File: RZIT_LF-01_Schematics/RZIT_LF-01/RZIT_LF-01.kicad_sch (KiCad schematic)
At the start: 0 parts

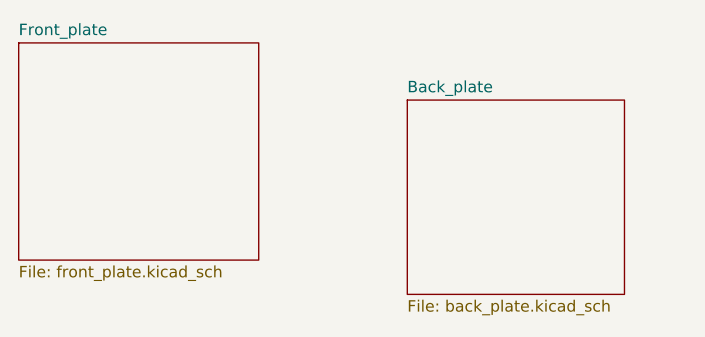
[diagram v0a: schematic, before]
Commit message: Changes
addetd
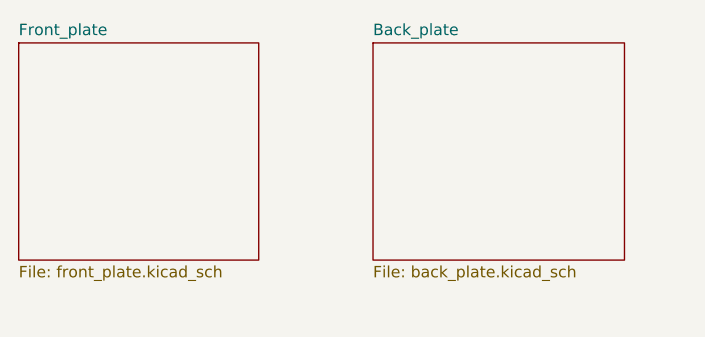
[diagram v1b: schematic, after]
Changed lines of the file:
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@@
 (kicad_sch (version 20211123) (generator eeschema)
   (paper "A4")
-  (sheet (at 118.11 54.61) (size 24.13 21.59) (fields_autoplaced)
+  (sheet (at 114.3 48.26) (size 27.94 24.13) (fields_autoplaced)
     (stroke (width 0.1524) (type solid) (color 0 0 0 0))
     (fill (color 0 0 0 0.0000))
-    (property "Sheet name" "Back_plate" (id 0) (at 118.11 53.8984 0)
+    (property "Sheet name" "Back_plate" (id 0) (at 114.3 47.5484 0)
       (effects (font (size 1.27 1.27)) (justify left bottom))
     )
-    (property "Sheet file" "back_plate.kicad_sch" (id 1) (at 118.11 76.7846 0)
+    (property "Sheet file" "back_plate.kicad_sch" (id 1) (at 114.3 72.9746 0)
       (effects (font (size 1.27 1.27)) (justify left top))
     )
@@
       (reference "#PWR?") (unit 1) (value "GND") (footprint "")
     )
+    (path "/2e1b8e48-0b26-4cf5-b4e7-1ce16b5ce0be/08574ea4-3686-4249-a3df-6a8f55c428f0"
+      (reference "#PWR?") (unit 1) (value "+3.3V") (footprint "")
+    )
     (path "/2e1b8e48-0b26-4cf5-b4e7-1ce16b5ce0be/08fac2eb-8669-4a36-b11c-7892fe3d12e2"
       (reference "#PWR?") (unit 1) (value "GND") (footprint "")
@@
       (reference "#PWR?") (unit 1) (value "+3.3V") (footprint "")
     )
+    (path "/2e1b8e48-0b26-4cf5-b4e7-1ce16b5ce0be/24ba3905-43ac-4e40-82e7-128d44942746"
+      (reference "#PWR?") (unit 1) (value "GND") (footprint "")
+    )
     (path "/2e1b8e48-0b26-4cf5-b4e7-1ce16b5ce0be/25eb344f-2e26-4af0-b9d7-c2dc91bae6a6"
       (reference "#PWR?") (unit 1) (value "GND") (footprint "")
@@
       (reference "#PWR?") (unit 1) (value "+3.3V") (footprint "")
     )
+    (path "/2e1b8e48-0b26-4cf5-b4e7-1ce16b5ce0be/30170b01-1124-4e99-90be-46e160dec4f3"
+      (reference "#PWR?") (unit 1) (value "GND") (footprint "")
+    )
     (path "/2e1b8e48-0b26-4cf5-b4e7-1ce16b5ce0be/31a9cdd2-5288-4d9b-bf4b-95e2dd897f61"
       (reference "#PWR?") (unit 1) (value "+3.3V") (footprint "")
@@
       (reference "#PWR?") (unit 1) (value "+3.3V") (footprint "")
     )
-    (path "/2e1b8e48-0b26-4cf5-b4e7-1ce16b5ce0be/a720cf76-448f-4fa9-b241-862453258760"
-      (reference "#PWR?") (unit 1) (value "GND") (footprint "")
-    )
     (path "/2e1b8e48-0b26-4cf5-b4e7-1ce16b5ce0be/a79bf299-ed19-4f53-9d17-c9f2e158af71"
       (reference "#PWR?") (unit 1) (value "GND") (footprint "")
@@
       (reference "#PWR?") (unit 1) (value "+3.3V") (footprint "")
     )
+    (path "/2e1b8e48-0b26-4cf5-b4e7-1ce16b5ce0be/d7035a7a-77eb-4ac5-a4a7-60dbe8fb1ef1"
+      (reference "C?") (unit 1) (value "100nF") (footprint "")
+    )
+    (path "/2e1b8e48-0b26-4cf5-b4e7-1ce16b5ce0be/f7f08f22-7201-41d0-b3e9-3d6d3862c50b"
+      (reference "C?") (unit 1) (value "4.7uF") (footprint "")
+    )
     (path "/2e1b8e48-0b26-4cf5-b4e7-1ce16b5ce0be/1c2dab5a-9a43-4cc0-b7fa-78917f8390f0"
       (reference "R?") (unit 1) (value "200") (footprint "")
@@
       (reference "R?") (unit 1) (value "20k") (footprint "")
     )
+    (path "/2e1b8e48-0b26-4cf5-b4e7-1ce16b5ce0be/3eee4add-1700-4e59-b90c-0c7ae537c501"
+      (reference "R?") (unit 1) (value "10k") (footprint "")
+    )
     (path "/2e1b8e48-0b26-4cf5-b4e7-1ce16b5ce0be/48d87eda-b5a7-4dd7-8482-e51be96f6a18"
       (reference "R?") (unit 1) (value "20k") (footprint "")
@@
       (reference "R?") (unit 1) (value "20k") (footprint "")
     )
+    (path "/2e1b8e48-0b26-4cf5-b4e7-1ce16b5ce0be/6031abde-b833-4f66-a1d6-40421ab3a37f"
+      (reference "R?") (unit 1) (value "10k") (footprint "")
+    )
     (path "/2e1b8e48-0b26-4cf5-b4e7-1ce16b5ce0be/72bb3040-bd09-4e3a-95bc-d3043bc9b4b7"
       (reference "R?") (unit 1) (value "200") (footprint "")
     )
+    (path "/2e1b8e48-0b26-4cf5-b4e7-1ce16b5ce0be/7ce0890a-dc24-451f-8dc3-ef0f4639c18f"
+      (reference "R?") (unit 1) (value "10k") (footprint "")
+    )
     (path "/2e1b8e48-0b26-4cf5-b4e7-1ce16b5ce0be/80299693-a029-4038-b7d8-5c94f629dc1d"
       (reference "R?") (unit 1) (value "20k") (footprint "")
@@
       (reference "R?") (unit 1) (value "200") (footprint "")
     )
+    (path "/2e1b8e48-0b26-4cf5-b4e7-1ce16b5ce0be/c12a6f96-6f0b-46b9-aaed-d5e718e4d3d6"
+      (reference "R?") (unit 1) (value "10k") (footprint "")
+    )
     (path "/2e1b8e48-0b26-4cf5-b4e7-1ce16b5ce0be/d2a58691-1ce2-4a44-b02d-e07298cb17d6"
       (reference "R?") (unit 1) (value "200") (footprint "")
@@
       (reference "U?") (unit 1) (value "QRE1113") (footprint "OptoDevice:OnSemi_CASE100AQ")
     )
-    (path "/2e1b8e48-0b26-4cf5-b4e7-1ce16b5ce0be/86eab7b8-2ba1-468f-aff8-8d00b048fda5"
+    (path "/2e1b8e48-0b26-4cf5-b4e7-1ce16b5ce0be/94c9a039-9b74-442a-be87-64ea896cb680"
+      (reference "U?") (unit 1) (value "QRE1113") (footprint "OptoDevice:OnSemi_CASE100AQ")
+    )
+    (path "/2e1b8e48-0b26-4cf5-b4e7-1ce16b5ce0be/9fa2dc80-2843-4c91-ad55-e90083707e05"
+      (reference "U?") (unit 1) (value "QRE1113") (footprint "OptoDevice:OnSemi_CASE100AQ")
+    )
+    (path "/2e1b8e48-0b26-4cf5-b4e7-1ce16b5ce0be/aac6220a-eaf7-46a5-9ea8-0cbd9e35573d"
+      (reference "U?") (unit 1) (value "QRE1113") (footprint "OptoDevice:OnSemi_CASE100AQ")
+    )
+    (path "/2e1b8e48-0b26-4cf5-b4e7-1ce16b5ce0be/b071f758-43b7-4959-8880-34eff15be8fa"
+      (reference "U?") (unit 1) (value "QRE1113") (footprint "OptoDevice:OnSemi_CASE100AQ")
+    )
+    (path "/2e1b8e48-0b26-4cf5-b4e7-1ce16b5ce0be/e4c2de01-8174-46d2-8769-fcbe800f2b70"
       (reference "U?") (unit 1) (value "VL53L1CXV0FY1") (footprint "Sensor_Distance:ST_VL53L1x")
     )
-    (path "/2e1b8e48-0b26-4cf5-b4e7-1ce16b5ce0be/94c9a039-9b74-442a-be87-64ea896cb680"
-      (reference "U?") (unit 1) (value "QRE1113") (footprint "OptoDevice:OnSemi_CASE100AQ")
-    )
-    (path "/2e1b8e48-0b26-4cf5-b4e7-1ce16b5ce0be/9fa2dc80-2843-4c91-ad55-e90083707e05"
-      (reference "U?") (unit 1) (value "QRE1113") (footprint "OptoDevice:OnSemi_CASE100AQ")
-    )
-    (path "/2e1b8e48-0b26-4cf5-b4e7-1ce16b5ce0be/aac6220a-eaf7-46a5-9ea8-0cbd9e35573d"
-      (reference "U?") (unit 1) (value "QRE1113") (footprint "OptoDevice:OnSemi_CASE100AQ")
-    )
-    (path "/2e1b8e48-0b26-4cf5-b4e7-1ce16b5ce0be/b071f758-43b7-4959-8880-34eff15be8fa"
-      (reference "U?") (unit 1) (value "QRE1113") (footprint "OptoDevice:OnSemi_CASE100AQ")
-    )
     (path "/2e1b8e48-0b26-4cf5-b4e7-1ce16b5ce0be/e6bd091a-1102-4950-af60-0d60abf26d28"

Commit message: small changes
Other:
- company: (none) -> Rzeszowska Grupa IT ~ Krzysztof Strzepek
- title: (none) -> RzIT Line Follower project
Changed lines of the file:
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@@
 (kicad_sch (version 20211123) (generator eeschema)
   (paper "A4")
+  (title_block
+    (title "RzIT Line Follower project")
+    (date "2022-05-31")
+    (rev "1.0")
+    (company "Rzeszowska Grupa IT ~ Krzysztof Strzepek")
+  )
   (sheet (at 114.3 48.26) (size 27.94 24.13) (fields_autoplaced)
     (stroke (width 0.1524) (type solid) (color 0 0 0 0))
@@
       (reference "#PWR0154") (unit 1) (value "GND") (footprint "")
     )
+    (path "/2e1b8e48-0b26-4cf5-b4e7-1ce16b5ce0be/163e6b8b-1e74-4ebe-a97e-70f5bb153174"
+      (reference "#PWR?") (unit 1) (value "GND") (footprint "")
+    )
+    (path "/1fd4466b-2ca1-45cb-aec7-19b4b61d12d2/30fd7273-12d2-4c5d-9e3e-36162b03862b"
+      (reference "#PWR?") (unit 1) (value "+7.5V") (footprint "")
+    )
+    (path "/1fd4466b-2ca1-45cb-aec7-19b4b61d12d2/40cae0cf-b06d-4c8e-8633-0b4b72457b8f"
+      (reference "#PWR?") (unit 1) (value "GND") (footprint "")
+    )
+    (path "/1fd4466b-2ca1-45cb-aec7-19b4b61d12d2/448d1762-7d23-46e8-bf43-233f169489f8"
+      (reference "#PWR?") (unit 1) (value "GND") (footprint "")
+    )
+    (path "/2e1b8e48-0b26-4cf5-b4e7-1ce16b5ce0be/6bbd90c6-fa9e-4b74-9dc6-7e50a5e8ab41"
+      (reference "#PWR?") (unit 1) (value "+7.5V") (footprint "")
+    )
+    (path "/1fd4466b-2ca1-45cb-aec7-19b4b61d12d2/95862df0-2ff4-4d14-8692-075f12e2fc2a"
+      (reference "#PWR?") (unit 1) (value "+7.5V") (footprint "")
+    )
+    (path "/1fd4466b-2ca1-45cb-aec7-19b4b61d12d2/ad8452fc-09d2-406f-ba9c-c6eba77655c3"
+      (reference "#PWR?") (unit 1) (value "GND") (footprint "")
+    )
+    (path "/2e1b8e48-0b26-4cf5-b4e7-1ce16b5ce0be/f17e8f04-60ed-4a03-b4b5-51633b961540"
+      (reference "#PWR?") (unit 1) (value "GND") (footprint "")
+    )
     (path "/2e1b8e48-0b26-4cf5-b4e7-1ce16b5ce0be/cab93a15-0bba-4dcb-9464-b535d0de5b4a"
       (reference "C?") (unit 1) (value "10uF") (footprint "")
@@
       (reference "D?") (unit 1) (value "LED") (footprint "")
     )
+    (path "/1fd4466b-2ca1-45cb-aec7-19b4b61d12d2/0af280ea-fd41-427d-9021-030dd563c52b"
+      (reference "J?") (unit 1) (value "52437-2471") (footprint "524372471")
+    )
     (path "/2e1b8e48-0b26-4cf5-b4e7-1ce16b5ce0be/1c1ceb41-a4b5-42b1-a76c-15eea2ca991b"
       (reference "J?") (unit 1) (value "52437-2471") (footprint "524372471")
     )
+    (path "/1fd4466b-2ca1-45cb-aec7-19b4b61d12d2/7cc88869-d8cd-46b6-9d5c-16c2e9deda35"
+      (reference "J?") (unit 1) (value "Conn_01x02") (footprint "Connector_JST:JST_XH_B2B-XH-AM_1x02_P2.50mm_Vertical")
+    )
     (path "/2e1b8e48-0b26-4cf5-b4e7-1ce16b5ce0be/1c2dab5a-9a43-4cc0-b7fa-78917f8390f0"
